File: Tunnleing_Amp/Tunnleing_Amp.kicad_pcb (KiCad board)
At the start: 4 copper layers, 20 x 20 mm, 11 parts, among them IC1 OPA928DT, J1 Conn_01x02_Pin

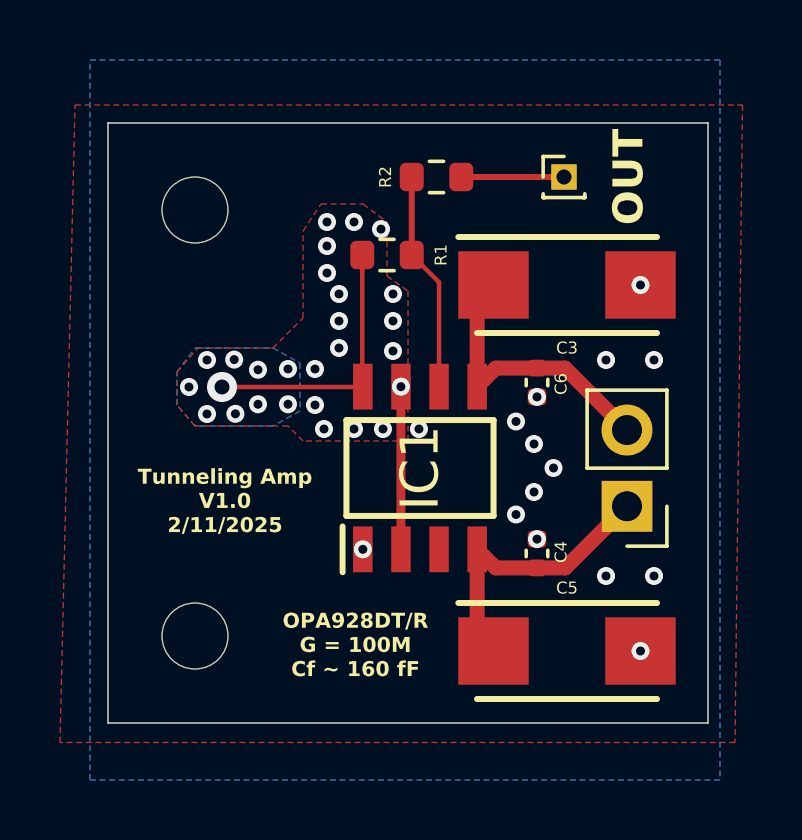
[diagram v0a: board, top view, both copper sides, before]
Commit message: Sent in V1.0 to JLC
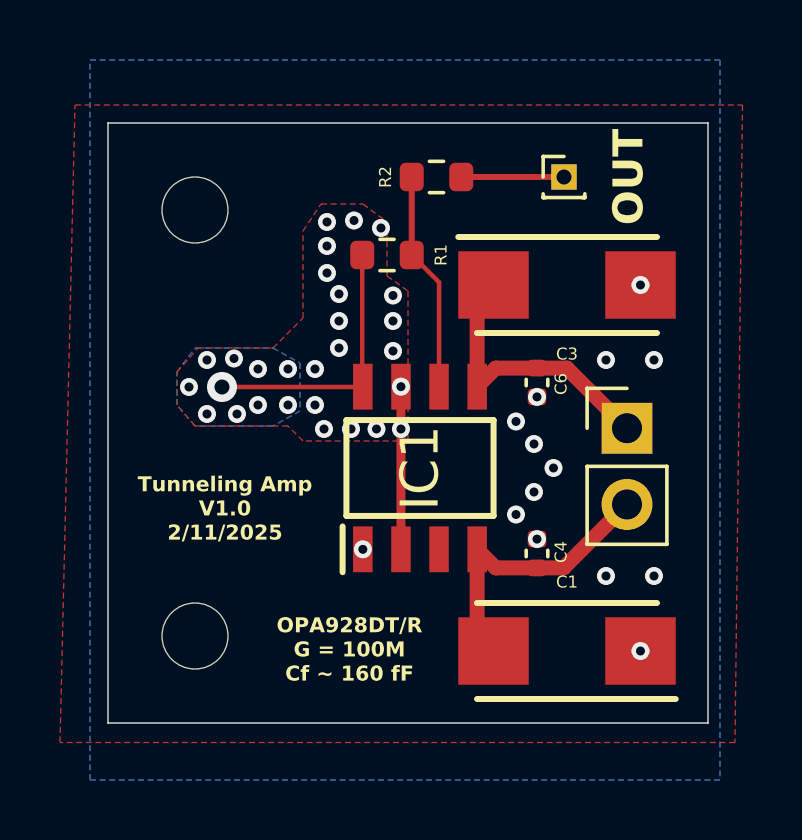
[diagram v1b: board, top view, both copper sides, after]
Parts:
- removed C5: 4.7uF, 293D475X9035C2TE3:CAPPM6032X280N
- added C1: 4.7uF, 293D475X9035C2TE3:CAPPM6032X280N, F.Cu at (106.9, 65.7)
- added G***: LOGO, LOGO, B.Cu at (101.4, 57.7)
- moved J1 2.60 mm to (108.9, 58.3), turned to 0 degrees
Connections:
- C3 pad 1: -15V -> +15V
- C4 pad 1: +15V -> -15V
- C6 pad 1: -15V -> +15V
- IC1 pad 2: GND -> /GRD
- IC1 pad 4: +15V -> -15V
- IC1 pad 5: -15V -> +15V
- IC1 pad 7: GND -> /GRD
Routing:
- net GND: track 5.42 -> 0.00 mm, vias 41 -> 14
- net /GRD: track 0.00 -> 5.42 mm, vias 0 -> 27
- added copper zone on B.Cu, net /GRD
- added copper zone on F.Cu, net /GRD
- added copper zone on In1.Cu, net /GRD
- added copper zone on In2.Cu, net /GRD
- removed copper zone on In1.Cu, net GND
- removed copper zone on In2.Cu, net GND
